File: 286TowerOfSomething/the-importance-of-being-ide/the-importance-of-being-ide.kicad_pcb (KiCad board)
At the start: 4 copper layers, 70 parts, among them J1 Bus_ISA_16bit, J2 Conn_02x20_Odd_Even, J3 Conn_02x20_Odd_Even, J4 IDE1_ACT, J5 IDE2_ACT, J6 IDE_ACT, SW1 SW_DIP_x08, U1 SST39SF010, U10 74ALS125, U11 74ALS125, U12 74ALS10, U13 74ALS688, U14 74LS07, U2 74ALS245, U3 74ALS245, U4 74ALS245, U5 74ALS245, U6 74ALS244, U7 GAL16V8, U8 74ALS138, U9 74ALS04

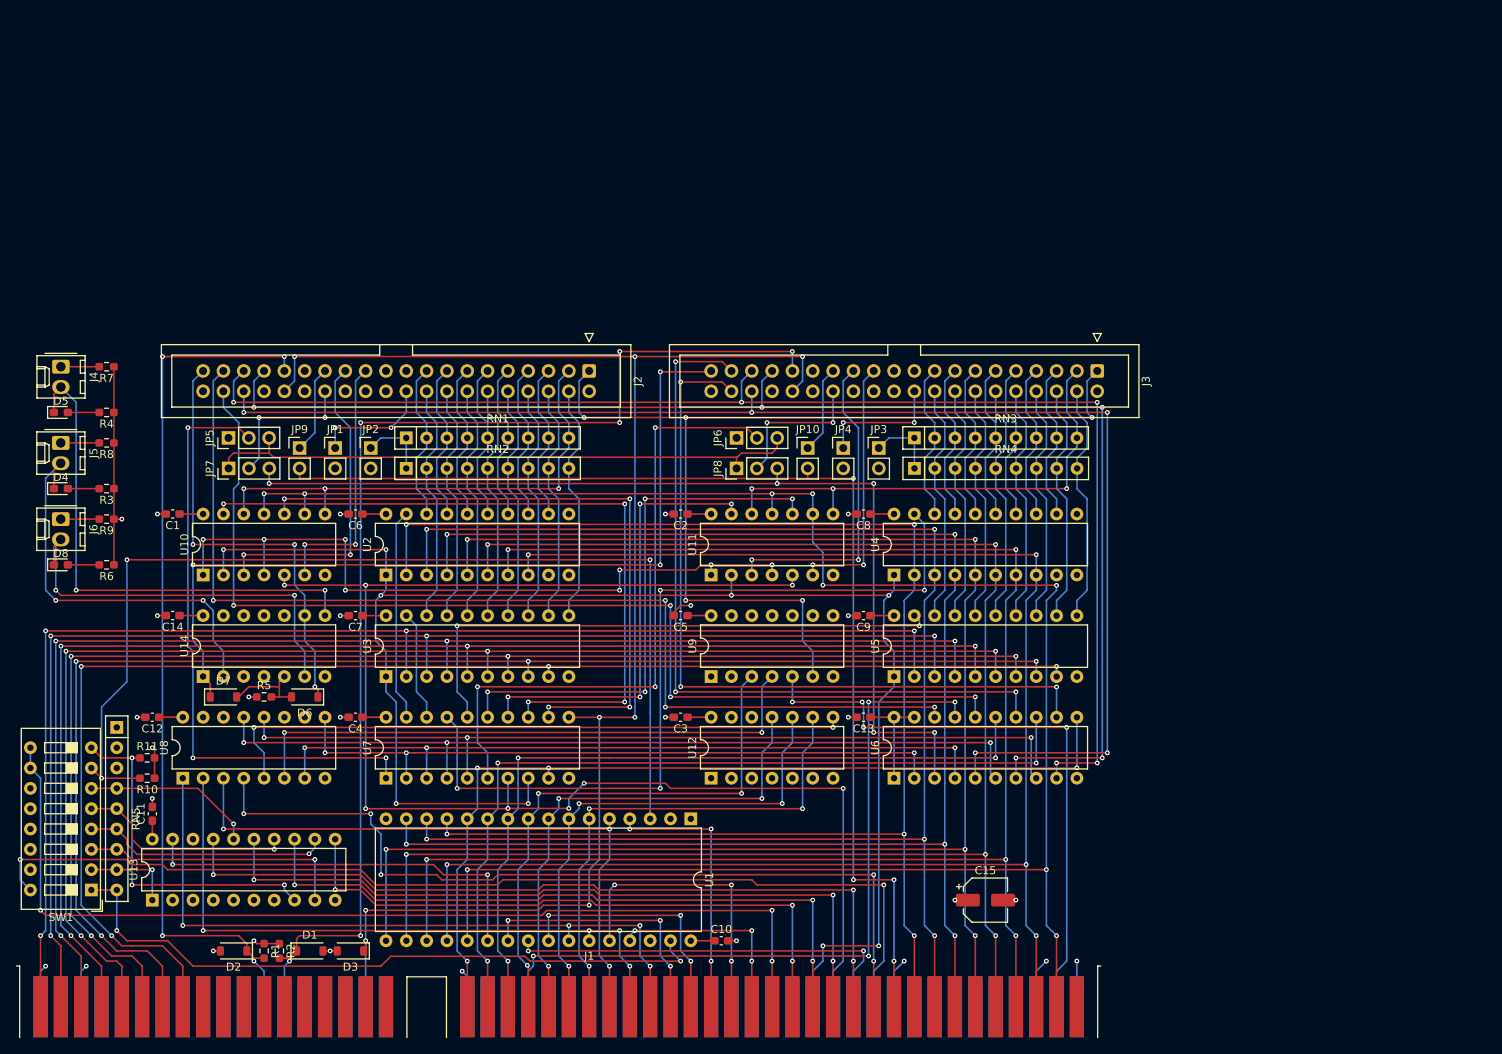
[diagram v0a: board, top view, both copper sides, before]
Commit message: Adding bracket to The Importance of Being IDE
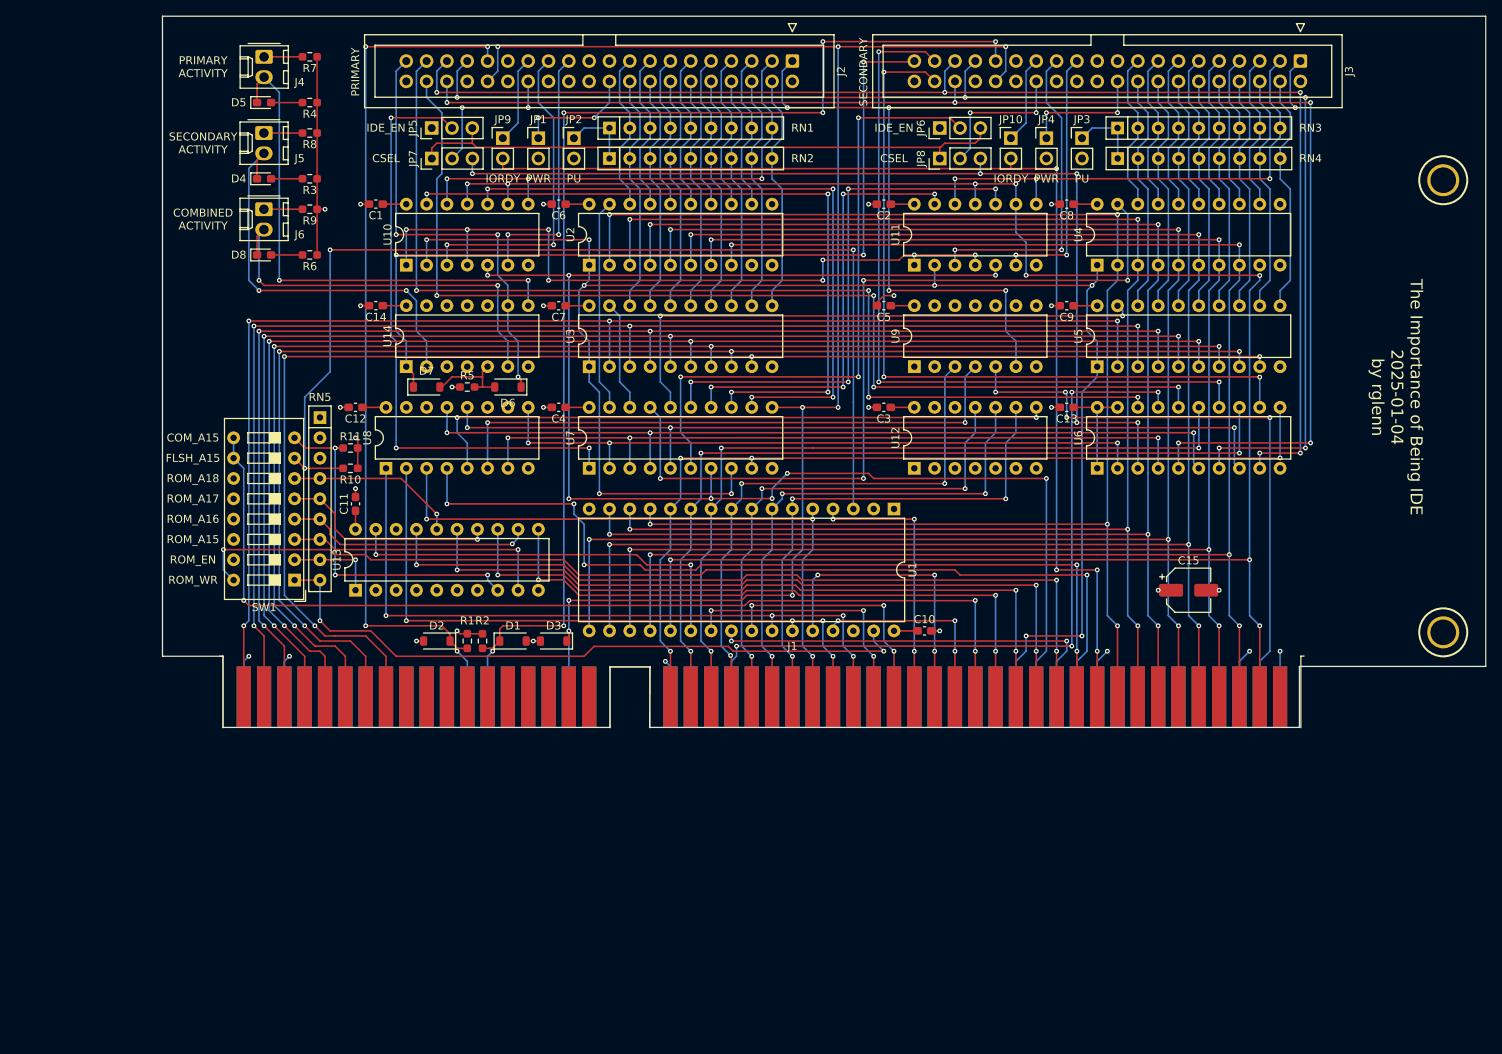
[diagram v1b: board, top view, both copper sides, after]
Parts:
- added BRACKET1: ~, pc-parts:PC_BRACKET_ISA_KEYSTONE_9202_Rev1, F.Cu at (190.5, 126.4)
- moved C15 46.3 mm to (179.1, 109.2)
- moved D2 46.3 mm to (85.1, 115.6)
- moved D6 46.3 mm to (94.0, 83.8)
- moved R1 46.3 mm to (88.9, 115.6)
- moved R2 46.3 mm to (90.8, 115.6)
- moved R5 46.3 mm to (88.9, 83.8)
- moved U13 46.3 mm to (74.9, 109.2)
- moved C10 46.3 mm to (146.1, 114.3)
- moved C11 46.3 mm to (74.9, 98.4)
- moved C12 46.3 mm to (74.9, 86.4)
- moved C13 46.3 mm to (163.8, 86.4)
- moved C3 46.3 mm to (141.0, 86.4)
- moved C5 46.3 mm to (141.0, 73.7)
- moved C9 46.3 mm to (163.8, 73.7)
- moved D1 46.3 mm to (94.6, 115.6)
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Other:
- board outline added: 165.4 x 88.9 mm
- board text added: "COMBINED ACTIVITY"
- board text added: "COM_A15"
- board text added: "CSEL"
- board text added: "FLSH_A15"
- board text added: "IDE_EN"
- board text added: "IORDY"
- board text added: "PRIMARY"
- board text added: "PRIMARY ACTIVITY"
- board text added: "PU"
- board text added: "PWR"
- board text added: "ROM_A15"
- board text added: "ROM_A16"
- board text added: "ROM_A17"
- board text added: "ROM_A18"
- board text added: "ROM_EN"
- board text added: "ROM_WR"
- board text added: "SECONDARY"
- board text added: "SECONDARY ACTIVITY"
- board text added: "The Importance of Being IDE 2025-01-04 by rglenn"
